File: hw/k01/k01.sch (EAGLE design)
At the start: 4 parts

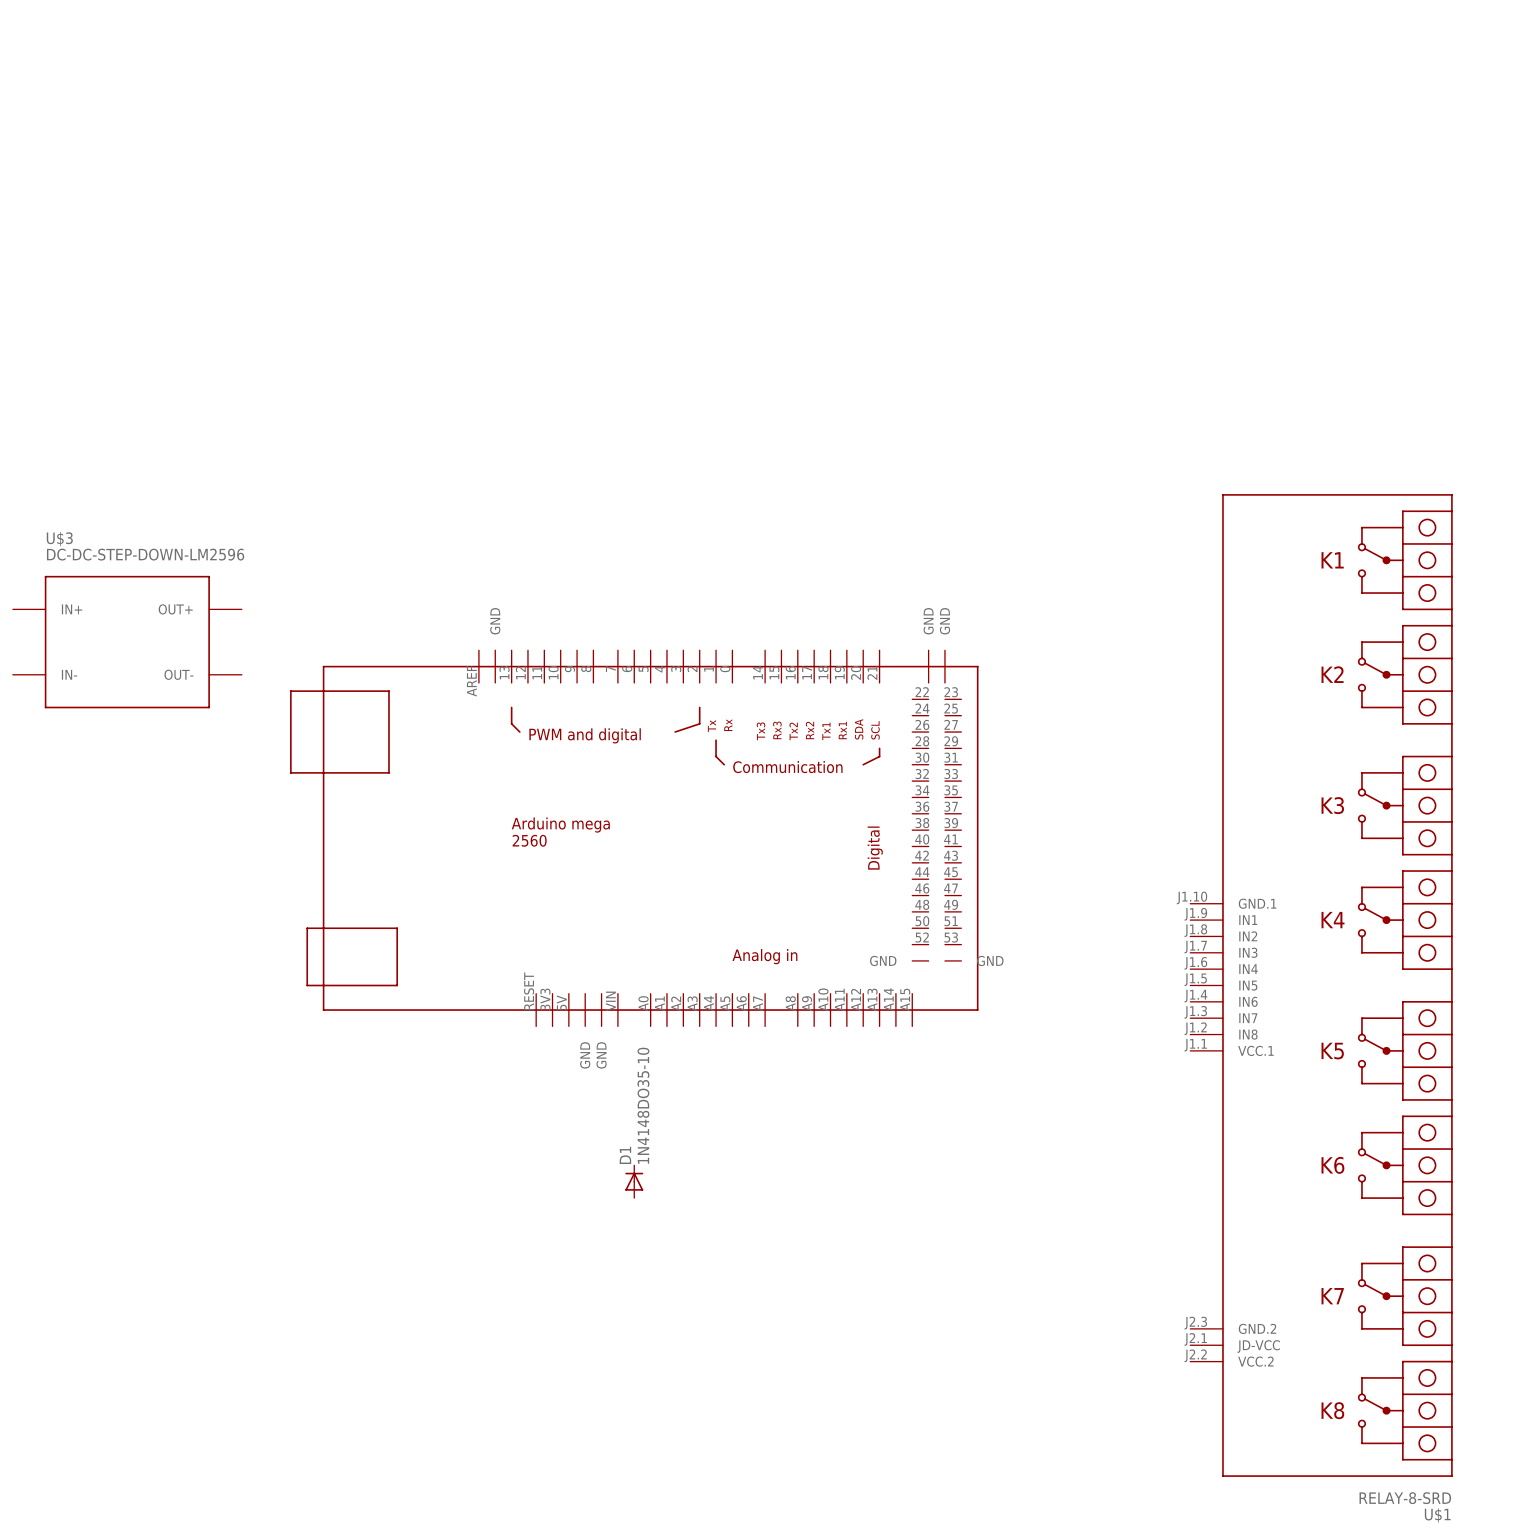
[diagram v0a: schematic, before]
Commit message: little updates 2
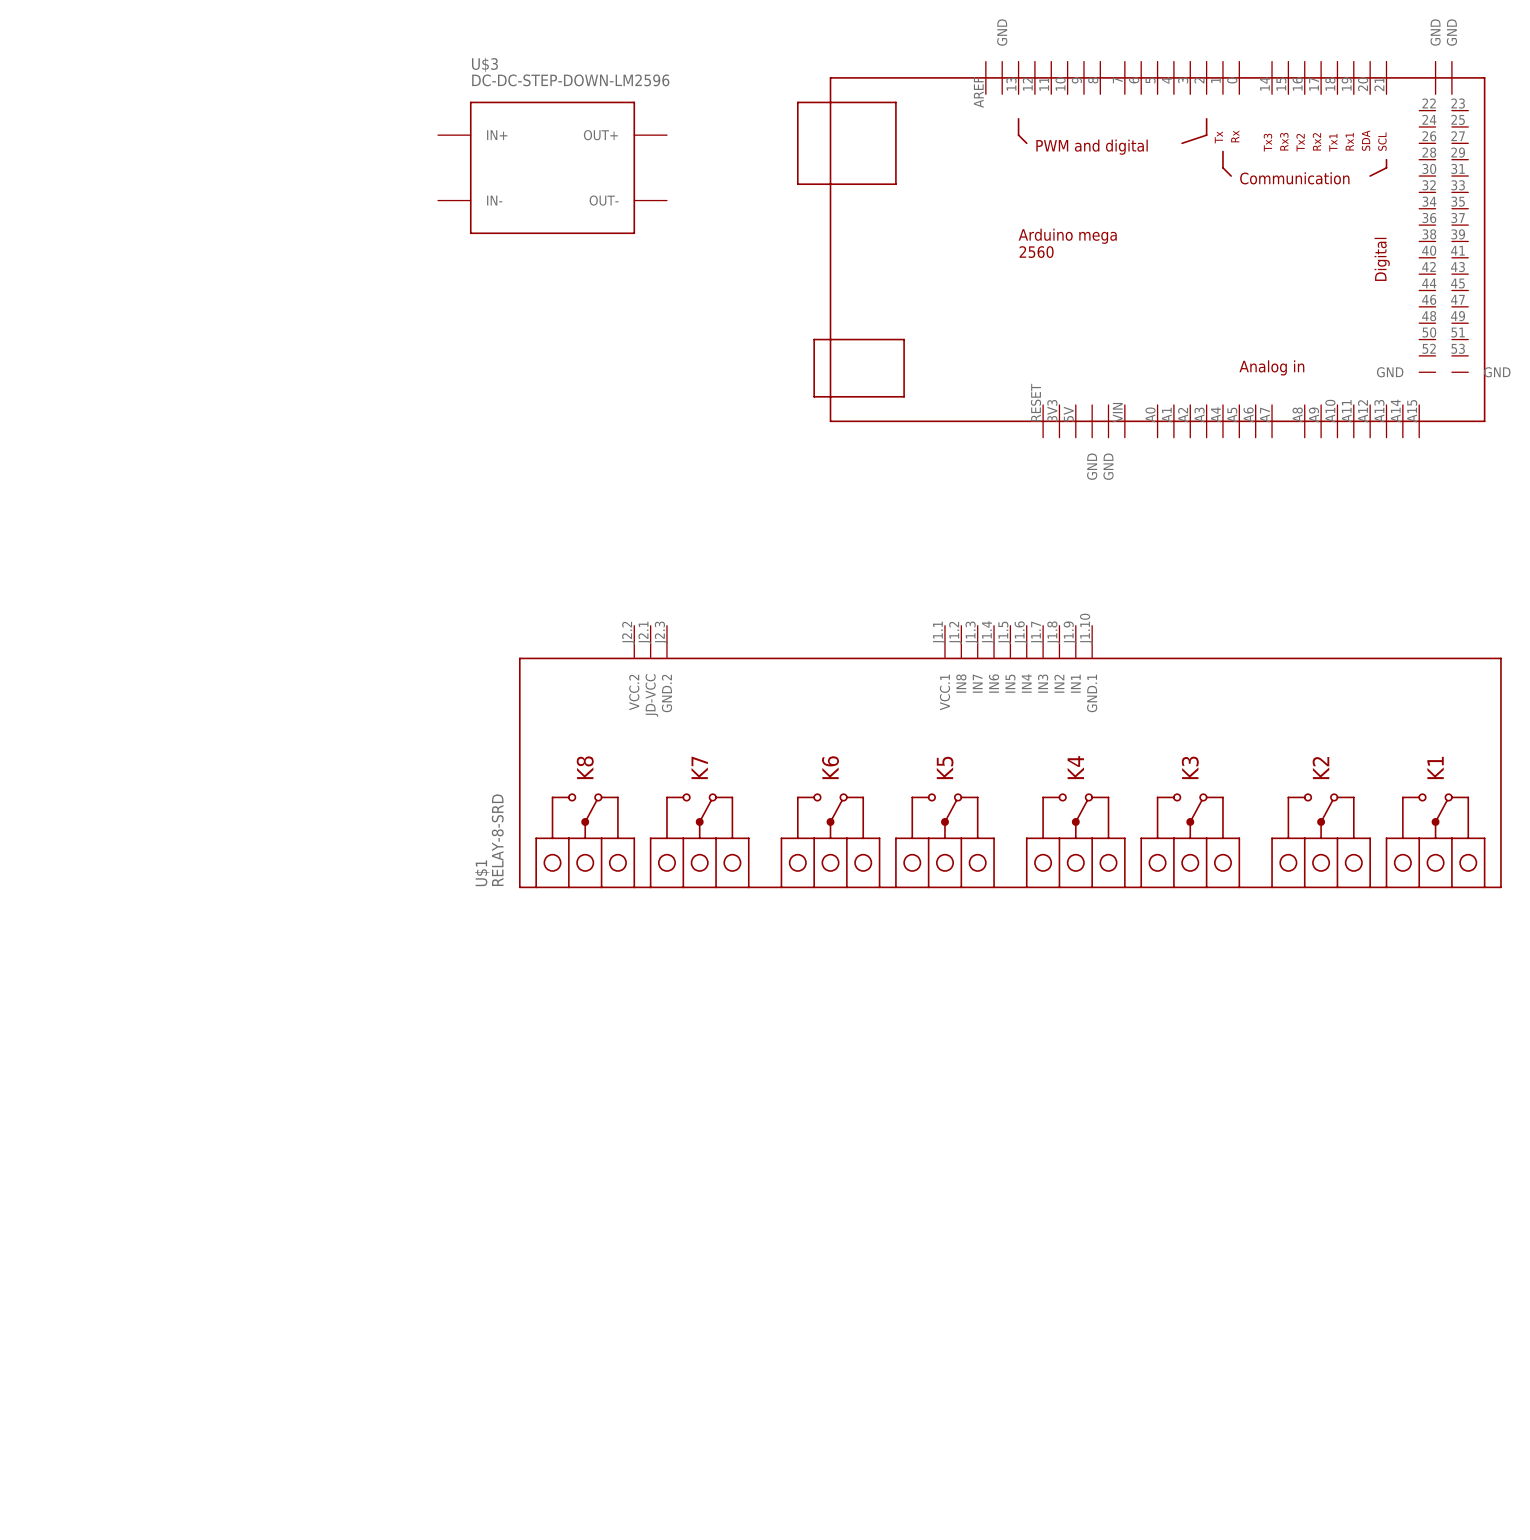
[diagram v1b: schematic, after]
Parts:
- removed D1: 1N4148DO35-10, diode:1N4148DO35-10
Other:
- moved on the sheet: U$1, U$3
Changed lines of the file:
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@@
 </classes>
 <parts>
-<part name="D1" library="diode" library_urn="urn:adsk.eagle:library:210" deviceset="1N4148" device="DO35-10" package3d_urn="urn:adsk.eagle:package:43344/2"/>
 <part name="U$1" library="diy-modules" deviceset="RELAY-8-SRD" device=""/>
 <part name="U$2" library="ArduinoMegaOutline" deviceset="MEGA_DEVICE" device=""/>
 <part name="U$3" library="diy-modules" deviceset="DC-DC-STEP-DOWN-LM2596" device=""/>
+<part name="FRAME1" library="frames" library_urn="urn:adsk.eagle:library:229" deviceset="A4L-LOC" device=""/>
 </parts>
 <sheets>
@@
 </plain>
 <instances>
-<instance part="D1" gate="G$1" x="55.88" y="-12.7" rot="R90"/>
-<instance part="U$1" gate="G$1" x="165.1" y="17.78" rot="R180"/>
-<instance part="U$2" gate="G$1" x="58.42" y="40.64"/>
-<instance part="U$3" gate="G$1" x="-22.86" y="71.12"/>
+<instance part="U$1" gate="G$1" x="114.3" y="50.8" rot="R90"/>
+<instance part="U$2" gate="G$1" x="137.16" y="132.08"/>
+<instance part="U$3" gate="G$1" x="43.18" y="144.78"/>
+<instance part="FRAME1" gate="G$1" x="0" y="0"/>
 </instances>
 <busses>
@@
 will not be understood (or retained) with this version.
 </note>
-<note version="8.3" severity="warning">
-Since Version 8.3, EAGLE supports the association of 3D packages
-with devices in libraries, schematics, and board files. Those 3D
-packages will not be understood (or retained) with this version.
-</note>
 </compatibility>
